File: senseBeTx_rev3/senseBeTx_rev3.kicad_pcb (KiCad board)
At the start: 2 copper layers, 32 x 60 mm, 41 parts, among them P1 CONN_02X05, Q1 SI2301, Q2 SI2302, Q3 SI2302, Q4 SI2302, SW1 Switch_SW_SPST, SW2 SW_Push_Dual, U1 STM32L011F3Px, U2 AP3403, Y1 Crystal

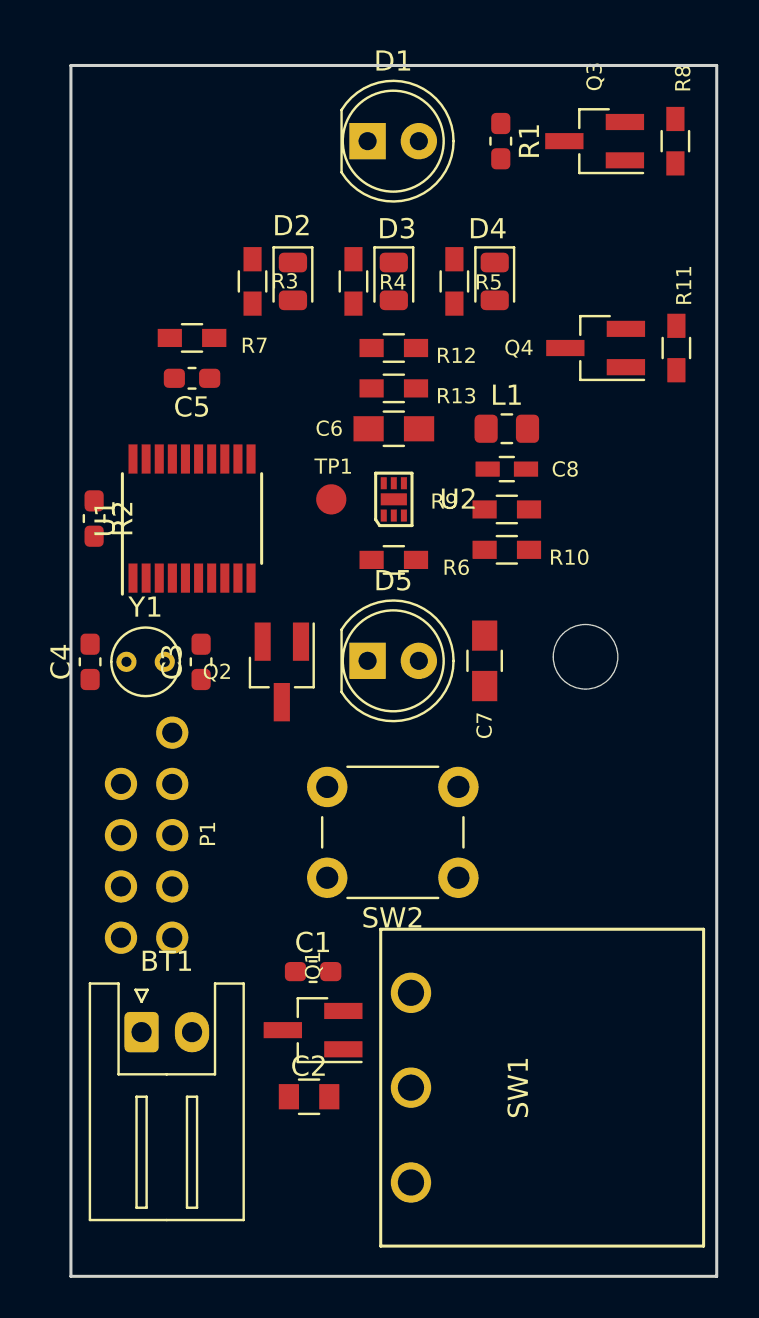
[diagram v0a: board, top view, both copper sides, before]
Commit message: Updates the local libraries.
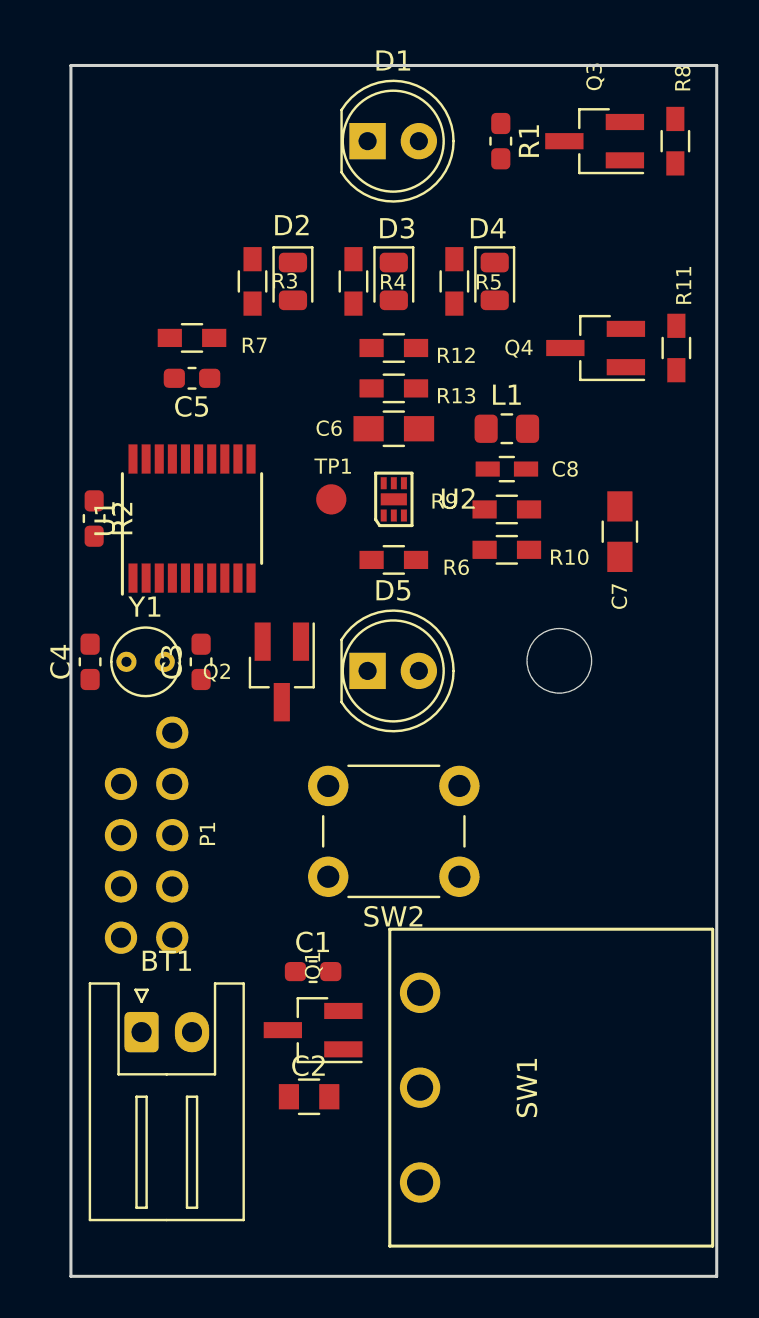
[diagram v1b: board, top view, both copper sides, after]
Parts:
- moved C7 9.27 mm to (42.5, 36.6)
- moved MK1 1.32 mm to (39.5, 43.0)
- moved D5 0.50 mm to (30.0, 43.5)
- moved SW1 0.45 mm to (32.6, 64.2)
- moved BT1 0.21 mm to (31.2, 43.0)
- moved SW2 0.07 mm to (34.5, 53.7)
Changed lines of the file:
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@@
   (general
     (thickness 1.6)
-    (drawings 8)
+    (drawings 13)
     (tracks 0)
     (zones 0)
@@
     (add_net VDD)
   )
+  (module senseBeTx_rev3_fp:2462_BatteryHolder_AAx2 locked (layer B.Cu)
+    (at 31.25 43)
+    (fp_text reference BT1 (at -0.01 30.45) (layer B.SilkS)
+      (effects (font (size 1 1) (thickness 0.15)) (justify mirror))
+    )
+    (fp_text value Battery (at 0 31.98) (layer B.Fab)
+      (effects (font (size 1 1) (thickness 0.15)) (justify mirror))
+    )
+    (fp_line (start 16.5 -29.5) (end -16.5 -29.5) (layer B.SilkS) (width 0.15))
+    (fp_line (start 16.5 29.5) (end 16.5 -29.5) (layer B.SilkS) (width 0.15))
+    (fp_line (start 16.5 29.5) (end -16.5 29.5) (layer B.SilkS) (width 0.15))
+    (fp_line (start -16.5 29.5) (end -16.5 -29.5) (layer B.SilkS) (width 0.15))
+    (model ${KIPRJMOD}/senseBeTx_rev3_3D_Files/C5404_AAx2_Battery_Holder.step
+      (at (xyz 0 0 0))
+      (scale (xyz 1 1 1))
+      (rotate (xyz 0 0 0))
+    )
+  )
   (module Connector_JST:JST_XH_S02B-XH-A_1x02_P2.50mm_Horizontal (layer F.Cu)
     (at 18.8 61.4)
@@
     )
   )
-  (module MountingHole:MountingHole_3.2mm_M3 (layer F.Cu)
-    (at 40.8 42.8)
+  (module MountingHole:MountingHole_3.2mm_M3 locked (layer F.Cu)
+    (at 39.5 43)
     (descr "Mounting Hole 3.2mm, no annular, M3")
     (tags "mounting hole 3.2mm no annular m3")
@@
     )
   )
-  (module senseBeTx_rev3_fp:2462_BatteryHolder_AAx2 locked (layer B.Cu)
-    (at 31.3 42.8)
-    (fp_text reference BT1 (at -0.01 30.45) (layer B.SilkS)
-      (effects (font (size 1 1) (thickness 0.15)) (justify mirror))
-    )
-    (fp_text value Battery (at 0 31.98) (layer B.Fab)
-      (effects (font (size 1 1) (thickness 0.15)) (justify mirror))
-    )
-    (fp_line (start 16.5 -29.5) (end -16.5 -29.5) (layer B.SilkS) (width 0.15))
-    (fp_line (start 16.5 29.5) (end 16.5 -29.5) (layer B.SilkS) (width 0.15))
-    (fp_line (start 16.5 29.5) (end -16.5 29.5) (layer B.SilkS) (width 0.15))
-    (fp_line (start -16.5 29.5) (end -16.5 -29.5) (layer B.SilkS) (width 0.15))
-    (model ${KIPRJMOD}/senseBeRx_rev3_3D_Files/C5404_AAx2_Battery_Holder.wrl
-      (at (xyz 0 0 0))
-      (scale (xyz 1 1 1))
-      (rotate (xyz 0 0 0))
-    )
-  )
   (module senseBeTx_rev3_fp:R_0603_HandSoldering (layer F.Cu)
     (at 34.3 24.2 90)
@@
   )
   (module senseBeTx_rev3_fp:C_0805_HandSoldering (layer F.Cu)
-    (at 35.8 43 90)
+    (at 42.5 36.6 90)
     (descr "Capacitor SMD 0805, hand soldering")
     (tags "capacitor 0805")
@@
   )
   (module LED_THT:LED_D5.0mm locked (layer F.Cu)
-    (at 30 43)
+    (at 30 43.5)
     (descr "LED, diameter 5.0mm, 2 pins, http://cdn-reichelt.de/documents/datenblatt/A500/LL-504BC2E-009.pdf")
     (tags "LED diameter 5.0mm 2 pins")
@@
   )
   (module senseBeTx_rev3_fp:SlideSwitch_1P2T_RightAngle (layer F.Cu)
-    (at 32.15 64.15 270)
+    (at 32.6 64.15 270)
     (fp_text reference SW1 (at 0 -5.33 270) (layer F.SilkS)
       (effects (font (size 1 1) (thickness 0.15)))
@@
   )
   (module Button_Switch_THT:SW_PUSH_6mm locked (layer F.Cu)
-    (at 34.5 53.75 180)
+    (at 34.55 53.7 180)
     (descr https://www.omron.com/ecb/products/pdf/en-b3f.pdf)
     (tags "tact sw push 6mm")
@@
     )
   )
+  (gr_line (start 48.8 43.5) (end 12.8 43.5) (layer Dwgs.User) (width 0.2))
+  (gr_line (start 48.8 13.5) (end 48.8 73.5) (layer Dwgs.User) (width 0.2))
+  (gr_line (start 31.3 74) (end 31.3 10) (layer Dwgs.User) (width 0.2))
+  (gr_line (start 31.3 74) (end 31.3 77) (layer Dwgs.User) (width 0.2))
+  (gr_line (start 15.3 74) (end 47.3 74) (layer Dwgs.User) (width 0.2))
   (gr_line (start 15.3 13.5) (end 15.3 73.5) (layer Margin) (width 0.2))
   (gr_line (start 47.3 13.5) (end 15.3 13.5) (layer Margin) (width 0.2))
